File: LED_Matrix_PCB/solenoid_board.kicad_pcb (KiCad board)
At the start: 2 copper layers, 103 parts, among them J2 MCU_LEFT_LEGS, J3 MCU_RIGHT_LEGS

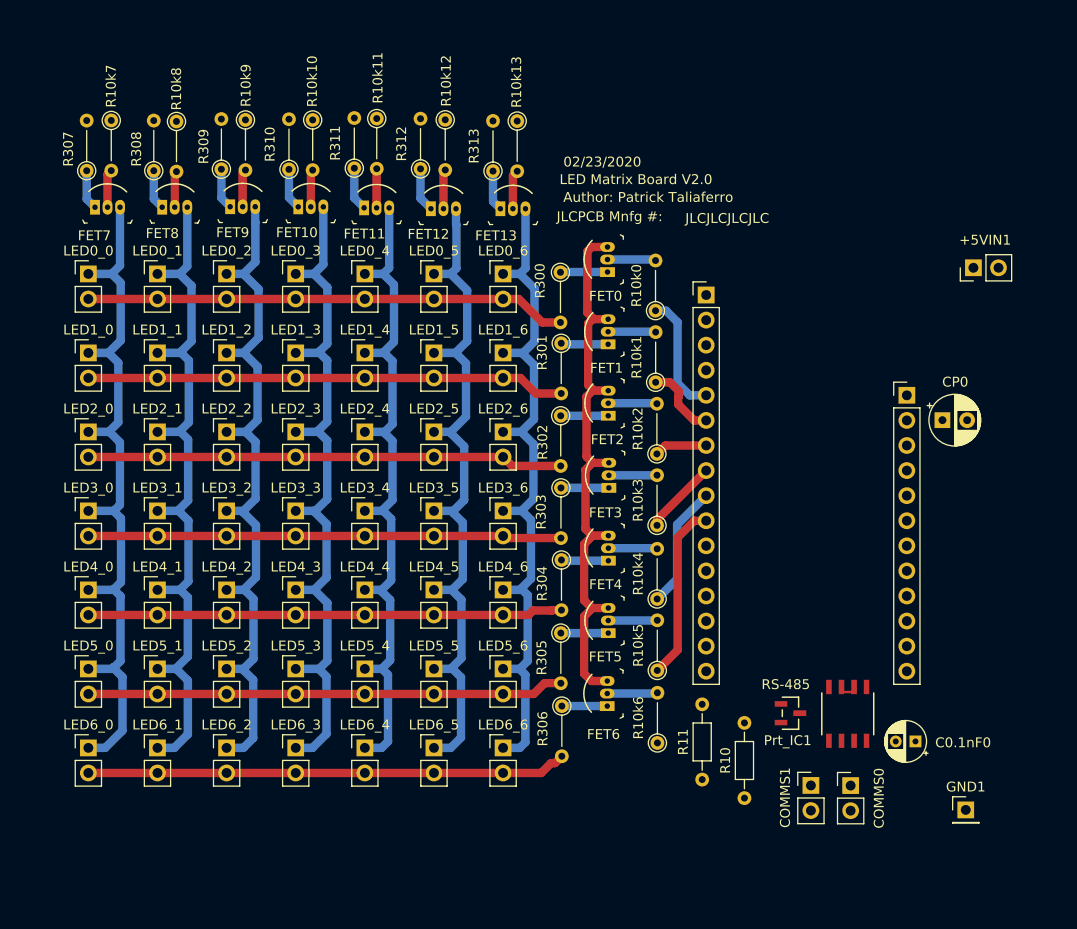
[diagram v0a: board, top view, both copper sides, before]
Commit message: Finished routing. Done. Ready to be merged. V2 Complete.
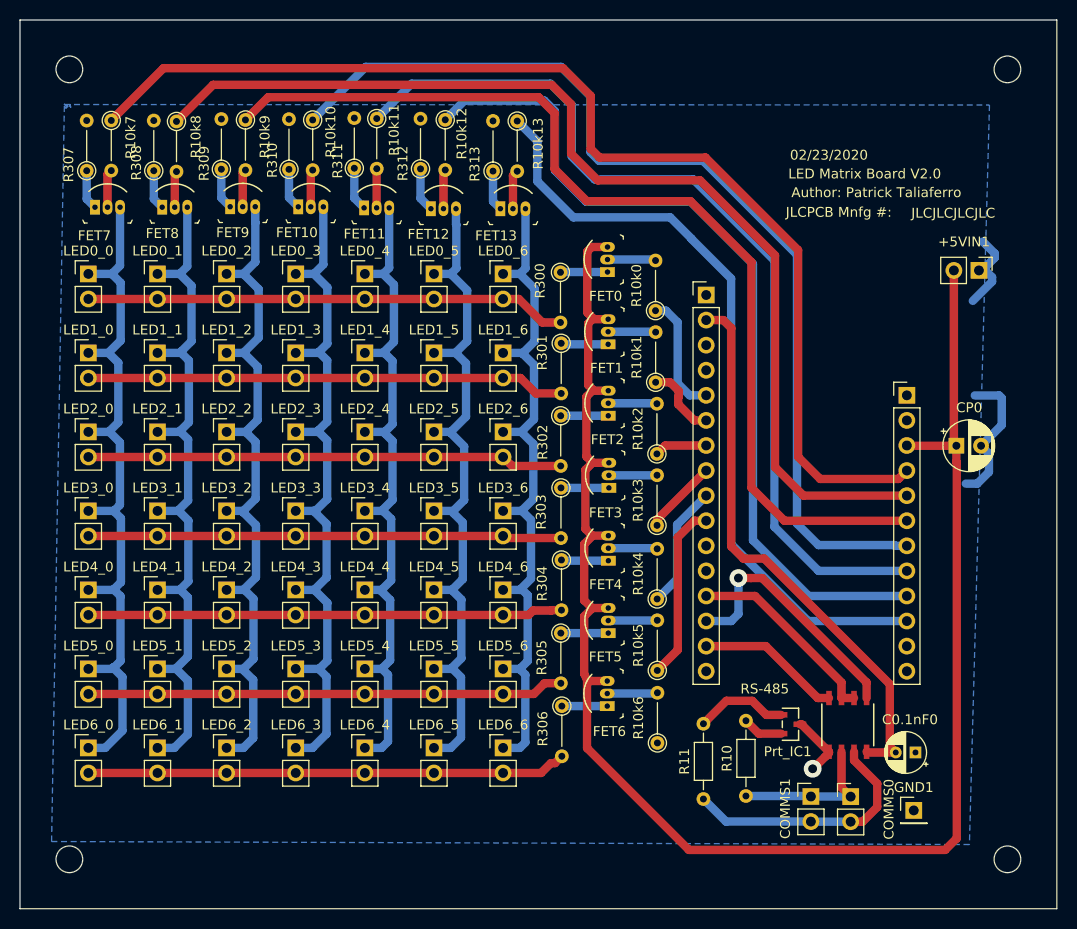
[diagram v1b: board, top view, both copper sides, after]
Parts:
- added REF**: MountingHole_2.7mm_M2.5, MountingHole:MountingHole_2.7mm_M2.5, F.Cu at (215.0, 135.0)
- added REF**: MountingHole_2.7mm_M2.5, MountingHole:MountingHole_2.7mm_M2.5, F.Cu at (215.0, 55.0)
- added REF**: MountingHole_2.7mm_M2.5, MountingHole:MountingHole_2.7mm_M2.5, F.Cu at (120.0, 55.0)
- added REF**: MountingHole_2.7mm_M2.5, MountingHole:MountingHole_2.7mm_M2.5, F.Cu at (120.0, 135.0)
- moved GND1 5.27 mm to (205.5, 130.0)
- moved CP0 2.95 mm to (209.8, 93.1)
- moved R11 1.97 mm to (184.2, 128.9)
- moved COMMS0 1.12 mm to (199.1, 128.7)
- moved C0.1nF0 1.12 mm to (205.7, 124.2)
- moved Prt_IC1 1.12 mm to (193.0, 121.3)
- moved RS-485 1.12 mm to (198.8, 121.4)
- moved COMMS1 1.12 mm to (195.1, 128.6)
- moved +5VIN1 0.62 mm to (212.1, 75.4), turned to 270 degrees
- moved R10 0.26 mm to (188.5, 128.6)
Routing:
- net /D13: track 0.00 -> 115.8 mm
- net +5V: track 58.5 -> 170.4 mm
- net /D12: track 0.00 -> 108.2 mm
- net /D11: track 0.00 -> 102.4 mm
- net /D10: track 0.00 -> 101.8 mm
- net /D9: track 0.00 -> 94.4 mm
- net /D6: track 0.00 -> 88.2 mm
- net /D5: track 0.00 -> 78.6 mm
- net +3V3: track 0.00 -> 57.0 mm
- net GND: track 0.00 -> 29.9 mm, vias 0 -> 1
- net /RX0: track 0.00 -> 26.1 mm, vias 0 -> 1
- net /B: track 0.00 -> 25.7 mm
- net /MISO: track 1.27 -> 20.2 mm
- net /A: track 0.00 -> 15.6 mm
- net /TX1: track 0.00 -> 14.6 mm
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- added copper zone on B.Cu, net GND
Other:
- board outline added: 105 x 90 mm
